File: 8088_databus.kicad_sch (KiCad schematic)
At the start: 3 parts, among them U16 74HC245

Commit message: fixes, prep for final production run
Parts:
- C33: LCSC Part # (none) -> C1853649
- RN4: LCSC Part # (none) -> C8692
- U16: LCSC Part # (none) -> C72118
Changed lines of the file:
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@@
 			)
 		)
-		(property "Description" "8 resistor network, star topology, bussed resistors, small symbol"
+		(property "Description" "LCSC #C8692 "
+			(at 227.33 101.6 0)
+			(effects
+				(font
+					(size 1.27 1.27)
+				)
+				(hide yes)
+			)
+		)
+		(property "Height" ""
+			(at 227.33 101.6 0)
+			(effects
+				(font
+					(size 1.27 1.27)
+				)
+				(hide yes)
+			)
+		)
+		(property "Manufacturer_Name" ""
+			(at 227.33 101.6 0)
+			(effects
+				(font
+					(size 1.27 1.27)
+				)
+				(hide yes)
+			)
+		)
+		(property "Manufacturer_Part_Number" ""
+			(at 227.33 101.6 0)
+			(effects
+				(font
+					(size 1.27 1.27)
+				)
+				(hide yes)
+			)
+		)
+		(property "Mouser Part Number" ""
+			(at 227.33 101.6 0)
+			(effects
+				(font
+					(size 1.27 1.27)
+				)
+				(hide yes)
+			)
+		)
+		(property "Mouser Price/Stock" ""
+			(at 227.33 101.6 0)
+			(effects
+				(font
+					(size 1.27 1.27)
+				)
+				(hide yes)
+			)
+		)
+		(property "LCSC Part #" "C8692 "
 			(at 227.33 101.6 0)
 			(effects
@@
 			)
 		)
-		(property "Description" ""
+		(property "Description" "LCSC #C1853649"
+			(at 148.59 78.74 0)
+			(effects
+				(font
+					(size 1.27 1.27)
+				)
+				(hide yes)
+			)
+		)
+		(property "Height" ""
+			(at 148.59 78.74 0)
+			(effects
+				(font
+					(size 1.27 1.27)
+				)
+				(hide yes)
+			)
+		)
+		(property "Manufacturer_Name" ""
+			(at 148.59 78.74 0)
+			(effects
+				(font
+					(size 1.27 1.27)
+				)
+				(hide yes)
+			)
+		)
+		(property "Manufacturer_Part_Number" ""
+			(at 148.59 78.74 0)
+			(effects
+				(font
+					(size 1.27 1.27)
+				)
+				(hide yes)
+			)
+		)
+		(property "Mouser Part Number" ""
+			(at 148.59 78.74 0)
+			(effects
+				(font
+					(size 1.27 1.27)
+				)
+				(hide yes)
+			)
+		)
+		(property "Mouser Price/Stock" ""
+			(at 148.59 78.74 0)
+			(effects
+				(font
+					(size 1.27 1.27)
+				)
+				(hide yes)
+			)
+		)
+		(property "LCSC Part #" "C1853649"
 			(at 148.59 78.74 0)
 			(effects
@@
 			)
 		)
-		(property "Description" ""
-			(at 139.7 101.6 0)
-			(effects
+		(property "Description" "LCSC #C72118 "
+			(at 139.7 101.6 0)
+			(effects
+				(font
+					(size 1.27 1.27)
+				)
+				(hide yes)
+			)
+		)
+		(property "Height" ""
+			(at 139.7 101.6 0)
+			(effects
+				(font
+					(size 1.27 1.27)
+				)
+				(hide yes)
+			)
+		)
+		(property "Manufacturer_Name" ""
+			(at 139.7 101.6 0)
+			(effects
+				(font
+					(size 1.27 1.27)
+				)
+				(hide yes)
+			)
+		)
+		(property "Manufacturer_Part_Number" ""
+			(at 139.7 101.6 0)
+			(effects
+				(font
+					(size 1.27 1.27)
+				)
+				(hide yes)
+			)
+		)
+		(property "Mouser Part Number" ""
+			(at 139.7 101.6 0)
+			(effects
+				(font
+					(size 1.27 1.27)
+				)
+				(hide yes)
+			)
+		)
+		(property "Mouser Price/Stock" ""
+			(at 139.7 101.6 0)
+			(effects
+				(font
+					(size 1.27 1.27)
+				)
+				(hide yes)
+			)
+		)
+		(property "LCSC Part #" "C72118 "
+			(at 139.7 101.6 0)
+			(effects

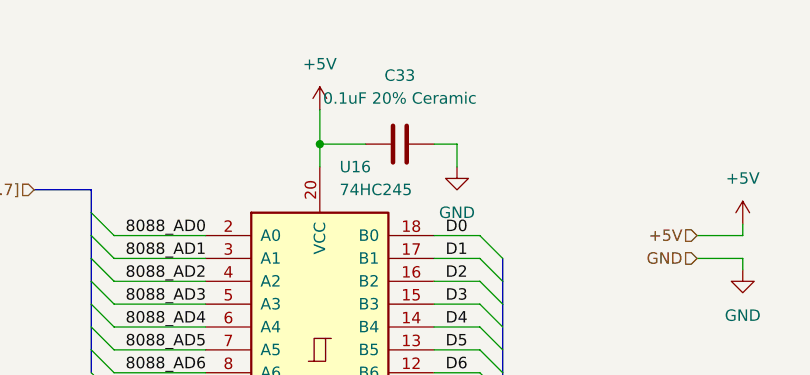
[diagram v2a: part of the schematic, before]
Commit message: no more SMT for isa_i2c, tweak motherboard multiplex logic, handful of other tweaks
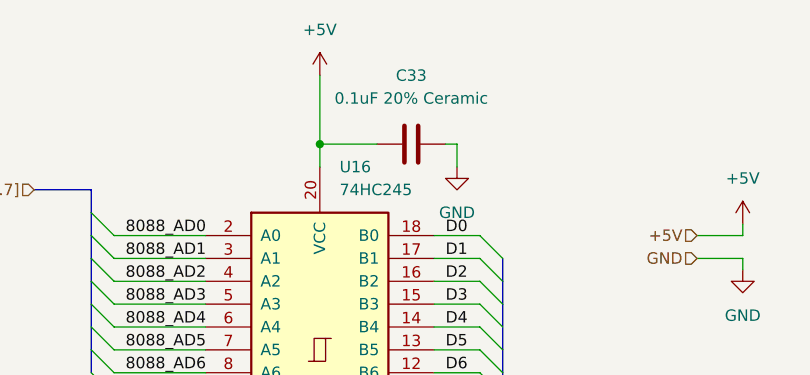
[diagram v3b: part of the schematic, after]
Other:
- moved on the sheet: C33
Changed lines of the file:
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@@
 	(wire
 		(pts
-			(xy 139.7 74.93) (xy 139.7 78.74)
+			(xy 139.7 71.12) (xy 139.7 78.74)
 		)
 		(stroke
@@
 	(wire
 		(pts
-			(xy 139.7 78.74) (xy 144.78 78.74)
+			(xy 139.7 78.74) (xy 146.05 78.74)
 		)
 		(stroke
@@
 	(wire
 		(pts
-			(xy 152.4 78.74) (xy 154.94 78.74)
+			(xy 153.67 78.74) (xy 154.94 78.74)
 		)
 		(stroke
@@
 	(symbol
 		(lib_id "Device:C")
-		(at 148.59 78.74 90)
+		(at 149.86 78.74 90)
 		(unit 1)
 		(exclude_from_sim no)
@@
 		(fields_autoplaced yes)
 		(property "Reference" "C33"
-			(at 148.59 71.12 90)
+			(at 149.86 71.12 90)
 			(effects
 				(font
@@
 		)
 		(property "Value" "0.1uF 20% Ceramic"
-			(at 148.59 73.66 90)
+			(at 149.86 73.66 90)
 			(effects
 				(font
@@
 		)
 		(property "Footprint" "Capacitor_SMD:C_0805_2012Metric"
-			(at 152.4 77.7748 0)
+			(at 153.67 77.7748 0)
 			(effects
 				(font
@@
 		)
 		(property "Datasheet" "~"
-			(at 148.59 78.74 0)
+			(at 149.86 78.74 0)
 			(effects
 				(font
@@
 		)
 		(property "Description" "LCSC #C1853649"
-			(at 148.59 78.74 0)
+			(at 149.86 78.74 0)
 			(effects
 				(font
@@
 		)
 		(property "Height" ""
-			(at 148.59 78.74 0)
+			(at 149.86 78.74 0)
 			(effects
 				(font
@@
 		)
 		(property "Manufacturer_Name" ""
-			(at 148.59 78.74 0)
+			(at 149.86 78.74 0)
 			(effects
 				(font
@@
 		)
 		(property "Manufacturer_Part_Number" ""
-			(at 148.59 78.74 0)
+			(at 149.86 78.74 0)
 			(effects
 				(font
@@
 		)
 		(property "Mouser Part Number" ""
-			(at 148.59 78.74 0)
+			(at 149.86 78.74 0)
 			(effects
 				(font
@@
 		)
 		(property "Mouser Price/Stock" ""
-			(at 148.59 78.74 0)
+			(at 149.86 78.74 0)
 			(effects
 				(font
@@
 		)
 		(property "LCSC Part #" "C1853649"
-			(at 148.59 78.74 0)
+			(at 149.86 78.74 0)
 			(effects
 				(font
@@
 	(symbol
 		(lib_id "power:+5V")
-		(at 139.7 74.93 0)
+		(at 139.7 71.12 0)
 		(unit 1)
 		(exclude_from_sim no)
@@
 		(fields_autoplaced yes)
 		(property "Reference" "#PWR054"
-			(at 139.7 78.74 0)
+			(at 139.7 74.93 0)
 			(effects
 				(font
@@
 		)
 		(property "Value" "+5V"
-			(at 139.7 69.85 0)
+			(at 139.7 66.04 0)
 			(effects
 				(font
@@
 		)
 		(property "Footprint" ""
-			(at 139.7 74.93 0)
+			(at 139.7 71.12 0)
 			(effects
 				(font
@@
 		)
 		(property "Datasheet" ""
-			(at 139.7 74.93 0)
+			(at 139.7 71.12 0)
 			(effects
 				(font
@@
 		)
 		(property "Description" ""
-			(at 139.7 74.93 0)
-			(effects
-				(font
+			(at 139.7 71.12 0)
+			(effects
+				(font
